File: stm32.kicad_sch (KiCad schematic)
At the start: 71 parts, among them J4 Conn_ST_STDC14, J5 Conn_02x20_Odd_Even, J7 TC2030 - TAG Connect, Q5 SI2301CDS-T1-GE3, SW1 SW_Push, SW2 SW_Push, U3 STM32F427V_G-I_Tx, X1 8MHz 20pF

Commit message: pre JLCPCB try 1
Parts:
- C11, C15, C16, C17, C30, C9: LCSC (none) -> C14663
- C12: LCSC C1525 -> C14663; Manufacturer Samsung -> (none)
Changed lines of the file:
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@@
 	(label "SPI3_SDO_*"
 		(at 186.69 212.09 0)
+		(fields_autoplaced yes)
 		(effects
 			(font
@@
 	(label "SPI3_SCK_*"
 		(at 186.69 207.01 0)
+		(fields_autoplaced yes)
 		(effects
 			(font
@@
 	(label "SPI3_SDI_*"
 		(at 186.69 209.55 0)
+		(fields_autoplaced yes)
 		(effects
 			(font
@@
 	(label "SPI2_CS_*"
 		(at 186.69 184.15 0)
+		(fields_autoplaced yes)
 		(effects
 			(font
@@
 	(label "SPI2_SDO_*"
 		(at 186.69 186.69 0)
+		(fields_autoplaced yes)
 		(effects
 			(font
@@
 			)
 		)
-		(property "LCSC" ""
+		(property "LCSC" "C14663"
 			(at 158.75 67.31 0)
 			(effects
@@
 			)
 		)
-		(property "LCSC" ""
+		(property "LCSC" "C14663"
 			(at 161.29 67.31 0)
 			(effects
@@
 			)
 		)
-		(property "LCSC" ""
+		(property "LCSC" "C14663"
 			(at 168.91 67.31 0)
 			(effects
@@
 			)
 		)
-		(property "LCSC" "C1525"
+		(property "LCSC" "C14663"
 			(at 163.83 67.31 0)
 			(effects
@@
 			)
 		)
-		(property "Manufacturer" "Samsung"
+		(property "Manufacturer" ""
 			(at 163.83 67.31 0)
 			(effects
@@
 			)
 		)
-		(property "LCSC" ""
+		(property "LCSC" "C14663"
 			(at 171.45 67.31 0)
 			(effects
@@
 			)
 		)
-		(property "LCSC" ""
+		(property "LCSC" "C14663"
 			(at 149.86 58.42 0)
 			(effects
@@
 			)
 		)
-		(property "LCSC" ""
+		(property "LCSC" "C14663"
 			(at 166.37 67.31 0)
 			(effects

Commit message: STM32 C117815
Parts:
- U3: LCSC (none) -> C117815
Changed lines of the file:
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@@
 			)
 		)
-		(property "LCSC" ""
+		(property "LCSC" "C117815"
 			(at 163.83 158.75 0)
 			(effects

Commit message: SENT TO jlcpcb
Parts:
- D11, D4, D5, D6: JLCPCB Rotation Offset (none) -> 180
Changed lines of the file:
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@@
+			)
+		)
+		(property "JLCPCB Rotation Offset" "180"
+			(at 314.96 105.41 0)
+			(effects
+				(font
+					(size 1.27 1.27)
+				)
+				(hide yes)
 			)
 		)
@@
 			)
 		)
+		(property "JLCPCB Rotation Offset" "180"
+			(at 314.96 113.03 0)
+			(effects
+				(font
+					(size 1.27 1.27)
+				)
+				(hide yes)
+			)
+		)
 		(pin "1"
 		)
@@
 			)
 		)
+		(property "JLCPCB Rotation Offset" "180"
+			(at 314.96 107.95 0)
+			(effects
+				(font
+					(size 1.27 1.27)
+				)
+				(hide yes)
+			)
+		)
 		(pin "1"
 		)
@@
 			(at 314.96 110.49 0)
 			(effects
+				(font
+					(size 1.27 1.27)
+				)
+				(hide yes)
+			)
+		)
+		(property "JLCPCB Rotation Offset" "180"
+			(at 314.96 110.49 0)
+			(effects

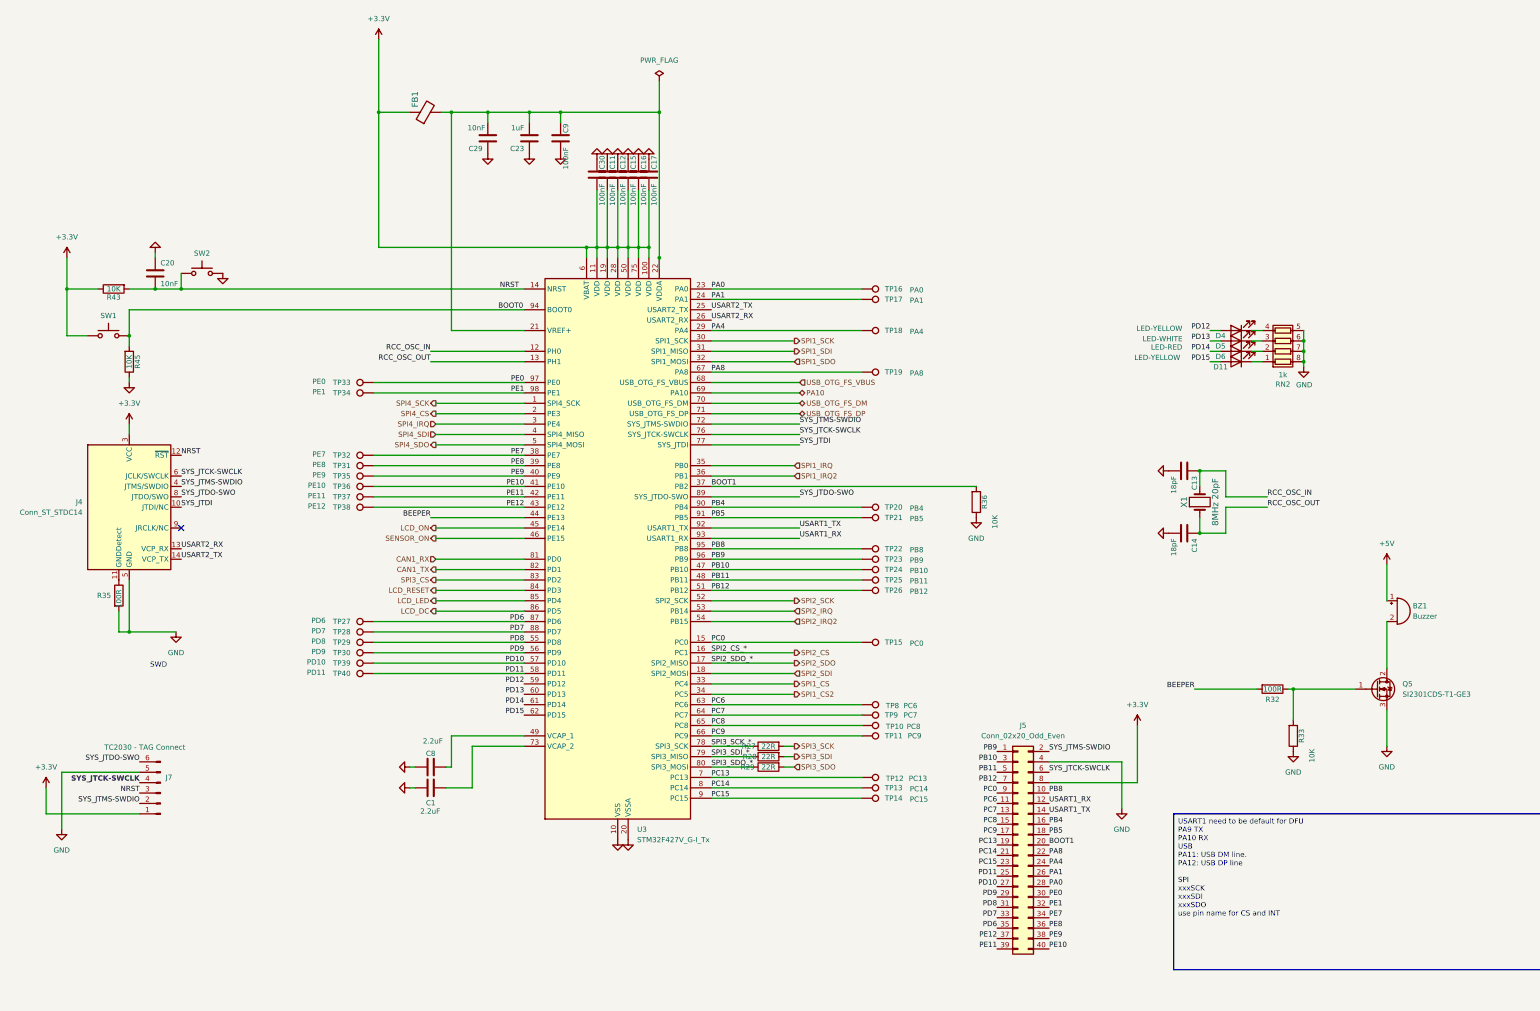
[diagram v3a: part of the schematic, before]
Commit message: version 2 changes
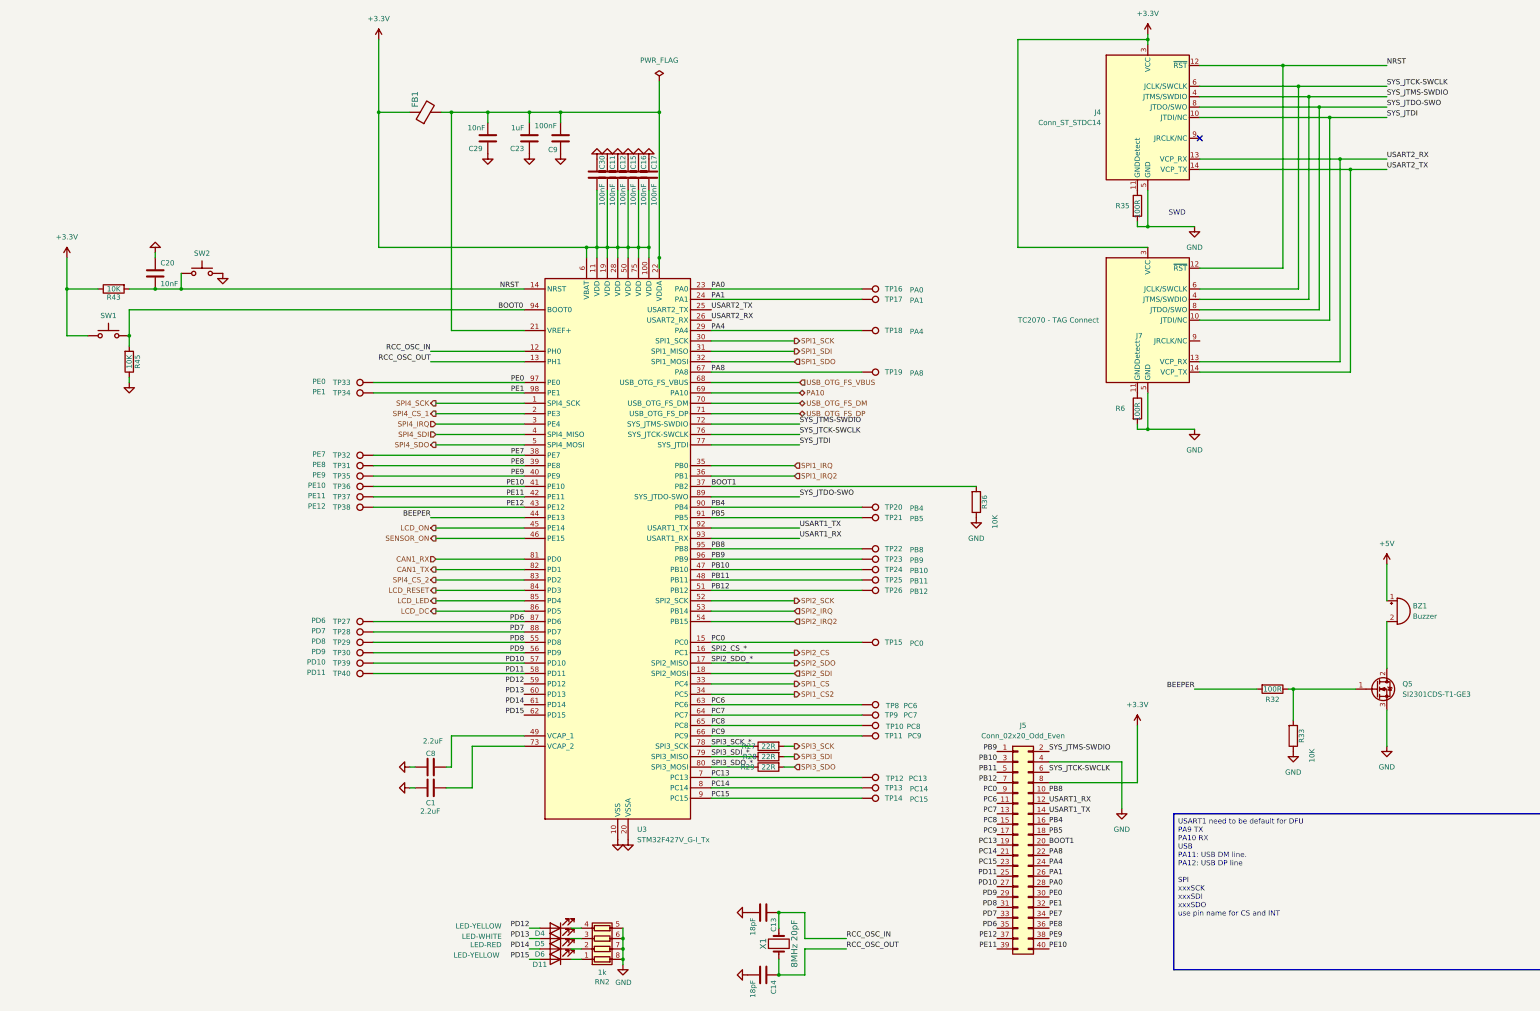
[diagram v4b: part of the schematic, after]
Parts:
- added R6: 100R, Resistor_SMD:R_0603_1608Metric, symbol Device:R
- FB1: symbol l8-kicad-rescue:Ferrite_Bead-Device -> Device:FerriteBead
- J4: footprint dnt:CON14_2X7_DUK_FTSH_SAI -> dnt:SAMTEC_FTSH-107-01-F-DV-K-Fix
- J7: value TC2030 - TAG Connect -> TC2070 - TAG Connect; footprint Connector:Tag-Connect_TC2030-IDC-NL_2x03_P1.27mm_Vertical -> Connector:Tag-Connect_TC2070-IDC-FP_2x07_P1.27mm_Vertical; symbol l8-kicad-rescue:Conn_01x06_Male-Connector -> Connector:Conn_ST_STDC14; now in the parts list
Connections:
- net +3.3V: now also J7.3 (VCC); no longer J7.1 (Pin_1)
- net GND: now also J7.7 (GND), R6.2
- net NRST: now also J7.12 (~{RST}); no longer J7.3 (Pin_3)
- net SYS_JTCK-SWCLK: now also J7.6 (JCLK/SWCLK); no longer J7.4 (Pin_4)
- net SYS_JTDI: now also J7.10 (JTDI/NC)
- net SYS_JTDO-SWO: now also J7.8 (JTDO/SWO); no longer J7.6 (Pin_6)
- net SYS_JTMS-SWDIO: now also J7.4 (JTMS/SWDIO); no longer J7.2 (Pin_2)
- net USART2_RX: now also J7.13 (VCP_RX)
- net USART2_TX: now also J7.14 (VCP_TX)
- net SPI3_CS renamed SPI4_CS_2
- net SPI4_CS renamed SPI4_CS_1
- new net: J7.11 (GNDDetect), R6.1
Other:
- moved on the sheet: C13, C14, D11, D4, D5, D6, J4, R35, RN2, X1
